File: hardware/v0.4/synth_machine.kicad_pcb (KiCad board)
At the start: 2 copper layers, 160 x 74 mm, 120 parts, among them J1 USB-C (MIDI + 5V power), J10 Pot VOL (10k lin, panel) JST-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, J15 STEMMA QT (I2C1), J16 Power switch (panel SPST) JST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, J17 Battery 1S LiPo (JST-PH, 1 = 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, J5 Speaker L (JST-PH), J6 Speaker R (JST-PH), J7 Headphones 3.5mm (CUI SJ1-351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, J8 Expansion, J9 Display (SPI1), K1 KEY C4 (direct D10) JST-XH, K10 A4 [c2 r2] JST-XH, K11 A#4 [c1 r1] JST-XH, K12 B4 [c1 r2] JST-XH, K13 C5 [c0 r2] JST-XH, K14 BTN1 [c0 r0] JST-XH, K15 BTN2 [c0 r1] JST-XH, K16 BTN3 [c1 r0] JST-XH, K17 BTN4 [c2 r0] JST-XH, K18 BTN5 [c3 r0] JST-XH, K19 BTN6 [c4 r0] JST-XH, K2 C#4 [c5 r0] JST-XH, K3 D4 [c5 r1] JST-XH, K4 D#4 [c4 r1] JST-XH, K5 E4 [c5 r2] JST-XH, K6 F4 [c4 r2] JST-XH, K7 F#4 [c3 r1] JST-XH, K8 G4 [c3 r2] JST-XH, K9 G#4 [c2 r1] JST-XH, Q1 2N7002, Q2 2N7002, U1 Daisy Seed / Seed3, U2 TPA6138A2PWR, U3 MAX98306ETD+T, U4 USBLC6-2SC6, U5 BQ24074RGTR, U6 TPS61023DRLR

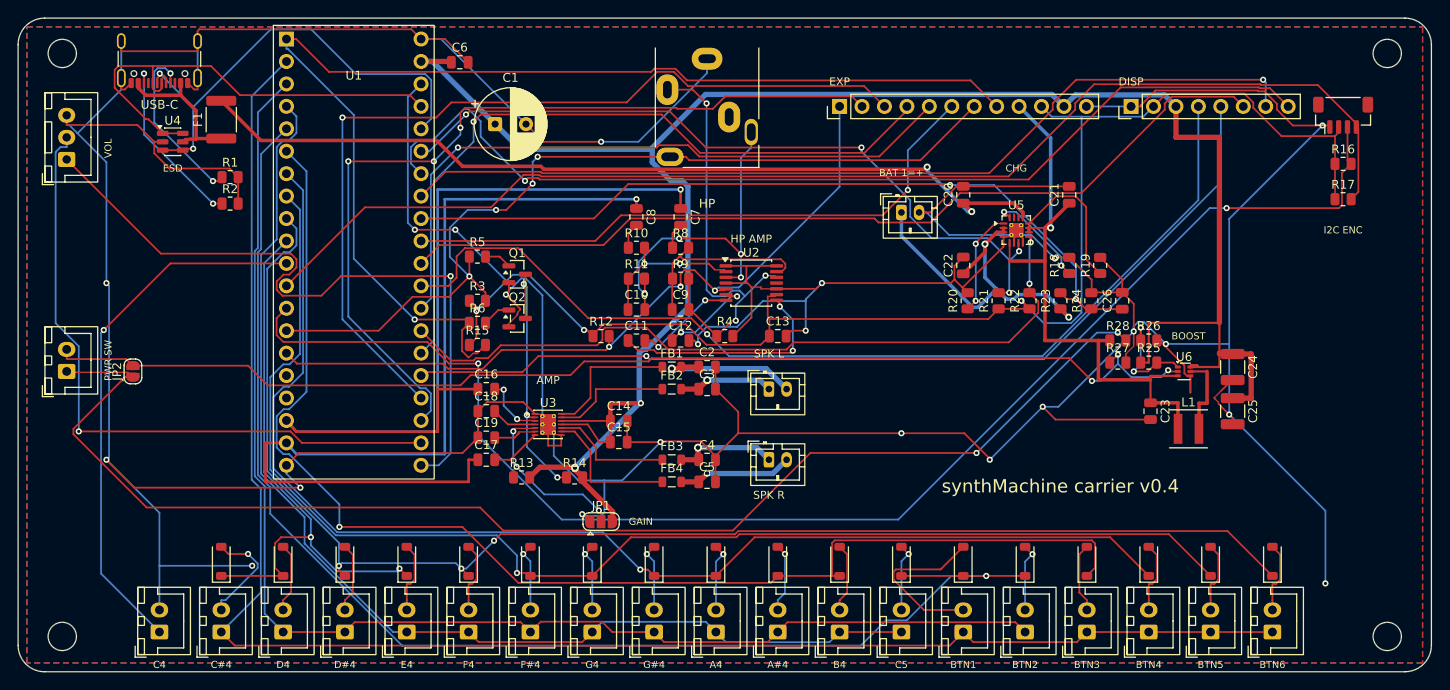
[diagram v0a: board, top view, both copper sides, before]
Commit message: Carrier v0.4: JP2 4 mm further from J16 so the PWR SW label reads
Co-Authored-By: Claude Fable 5.1 <noreply@anthropic.com>
Claude-Session: https://claude.ai/code/session_019ZDGV5fm4G7LwUwRWHEiwx
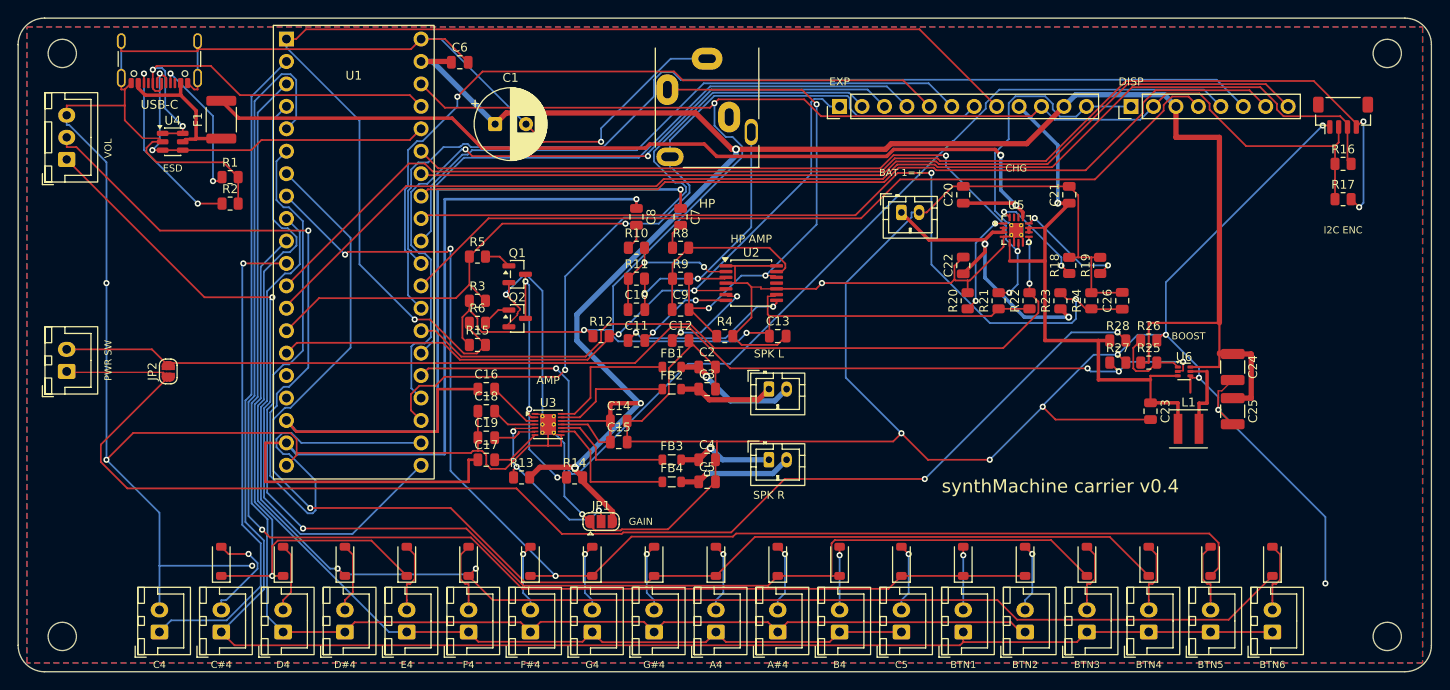
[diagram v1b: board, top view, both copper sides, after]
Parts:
- moved JP2 4.00 mm to (17.0, 40.0)
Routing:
- net +3V3: track 188.5 -> 232.4 mm, vias 5 -> 3
- net I2C_SDA: track 161.8 -> 137.7 mm, vias 2 -> 0
- net POT_VOL: track 74.6 -> 96.7 mm
- net SPI_SCK: track 114.2 -> 97.7 mm, vias 1 -> 0
- net EXP_A2: track 100.6 -> 86.7 mm, vias 1 -> 2
- net EXP_A1: track 97.3 -> 83.8 mm, vias 3 -> 1
- net SPI_MOSI: track 108.5 -> 120.9 mm
- net USB_DM: track 55.2 -> 43.1 mm
- net KBTN1_D: track 19.3 -> 7.15 mm, vias 0 -> 1
- net SPI_NSS: track 102.1 -> 113.2 mm
- net DISP_RST: track 114.4 -> 103.8 mm, vias 1 -> 0
- net HP_L: track 50.0 -> 58.8 mm
- net VBAT_SENSE: track 91.1 -> 99.6 mm
- net EXP_A6: track 76.3 -> 83.8 mm
- net VBAT: track 42.1 -> 35.1 mm
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
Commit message: Carrier v0.4: quality pass on current paths and the boost cluster
Audit of every current-carrying net on the routed board, and fixes:
- Boost converter (SOT-563, 0.5 mm pitch rows at y 39.5/40.0/40.5): 0.3 mm
  necks off VIN/SW/VOUT/GND no longer than the pitch forces, then 0.6 mm
  into the input cap, the inductor and the output cap. Previously 0.25 mm
  for several millimetres in series with the whole battery current.
- MAX98306 PVDD pins joined right off the pads into one 0.5 mm feed; the
  four speaker lines widen to 0.4 mm as soon as they separate. Previously
  0.2 mm for the full 6 to 15 mm runs.
- +5V trunk hand-routed on both layers from the boost to the display and
  expansion headers, down between the headphone amp and the speaker
  connectors to the amp's supply, and under the jack pads on B.Cu to the
  bulk cap at the Seed's VIN. The router had been leaving a different gap
  on this net each run. Power-class (0.5 mm drill) vias throughout; the
  pre-route via helper now takes a drill size.
- FB divider resistors stood on end so the FB node is a short diagonal and
  no +5V track threads between their pads.
- Checked and documented: the TPS61023 truly disconnects in shutdown (the
  panel switch does turn everything off), 470 uF is inside its output-cap
  range, boost thermals, the Seed 3V3 budget with encoder LEDs, USB-C
  current advertisement, the ADC divider impedance, reverse-cell and
  quiescent current. Notes in the v0.4 README.
Result: DRC 0 unconnected, ERC clean.

Co-Authored-By: Claude Fable 5.1 <noreply@anthropic.com>
Claude-Session: https://claude.ai/code/session_019ZDGV5fm4G7LwUwRWHEiwx
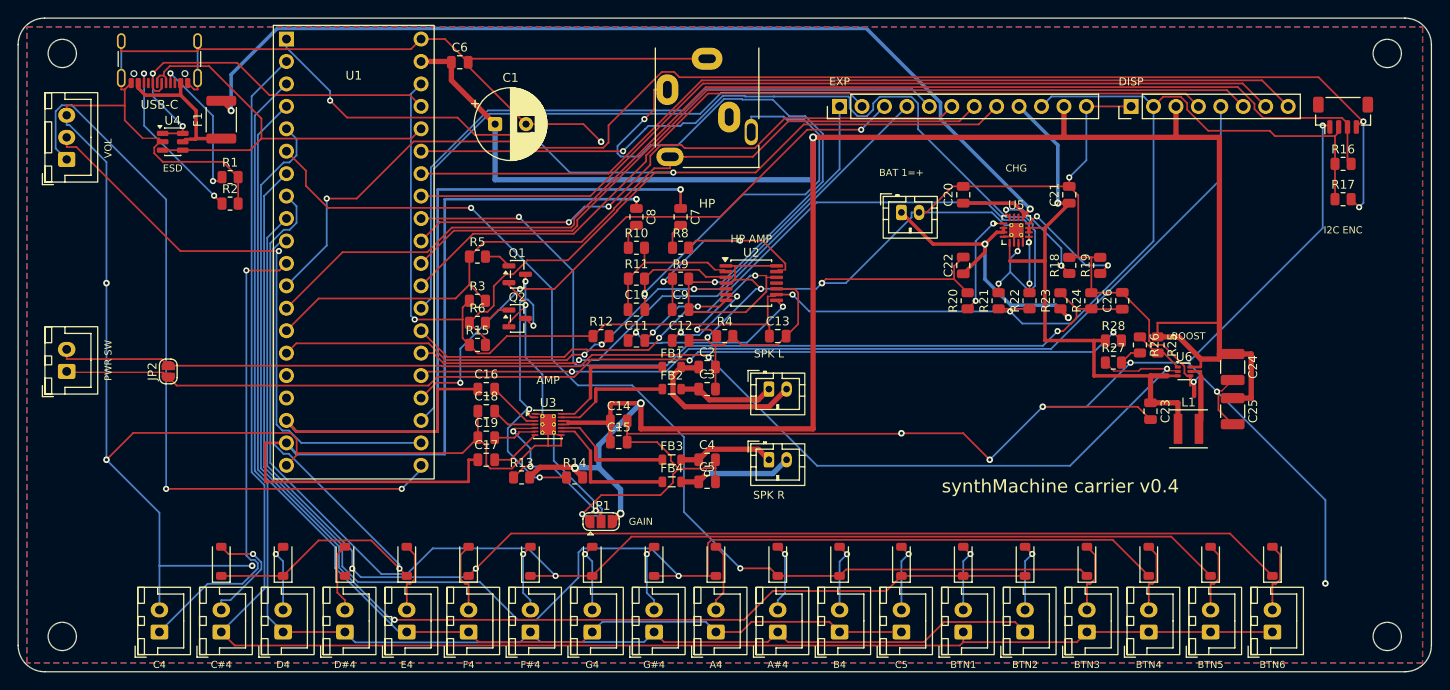
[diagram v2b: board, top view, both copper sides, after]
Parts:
- moved R25 2.24 mm to (129.0, 37.0), turned to -90 degrees
- moved R26 1.12 mm to (127.0, 37.0), turned to -90 degrees
- moved R27 0.50 mm to (124.0, 39.0)
- moved R28 0.50 mm to (124.0, 36.5)
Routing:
- net +3V3: track 232.4 -> 192.9 mm
- net HP_L: track 58.8 -> 92.7 mm, vias 3 -> 4
- net SW_HI: track 153.8 -> 123.1 mm
- net POT_VOL: track 96.7 -> 67.0 mm
- net COL1: track 146.8 -> 121.8 mm, vias 1 -> 2
- net +5V: track 242.2 -> 265.4 mm, vias 3 -> 4
- net HP_R: track 32.7 -> 54.2 mm, vias 2 -> 1
- net EXP_A2: track 86.7 -> 68.4 mm, vias 2 -> 3
- net USB_PGOOD: track 82.3 -> 100.0 mm
- net COL0: track 151.4 -> 138.0 mm
- net SPI_MOSI: track 120.9 -> 108.0 mm
- net GND: track 691.0 -> 679.8 mm, vias 16 -> 18
- net EXP_A4: track 78.6 -> 67.5 mm, vias 0 -> 1
- net SPI_NSS: track 113.2 -> 102.4 mm
- net VUSB: track 106.0 -> 116.7 mm
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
